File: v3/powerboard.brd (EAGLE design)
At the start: 100 x 80 mm, 17 parts, among them U1 TPS61088VQFN20

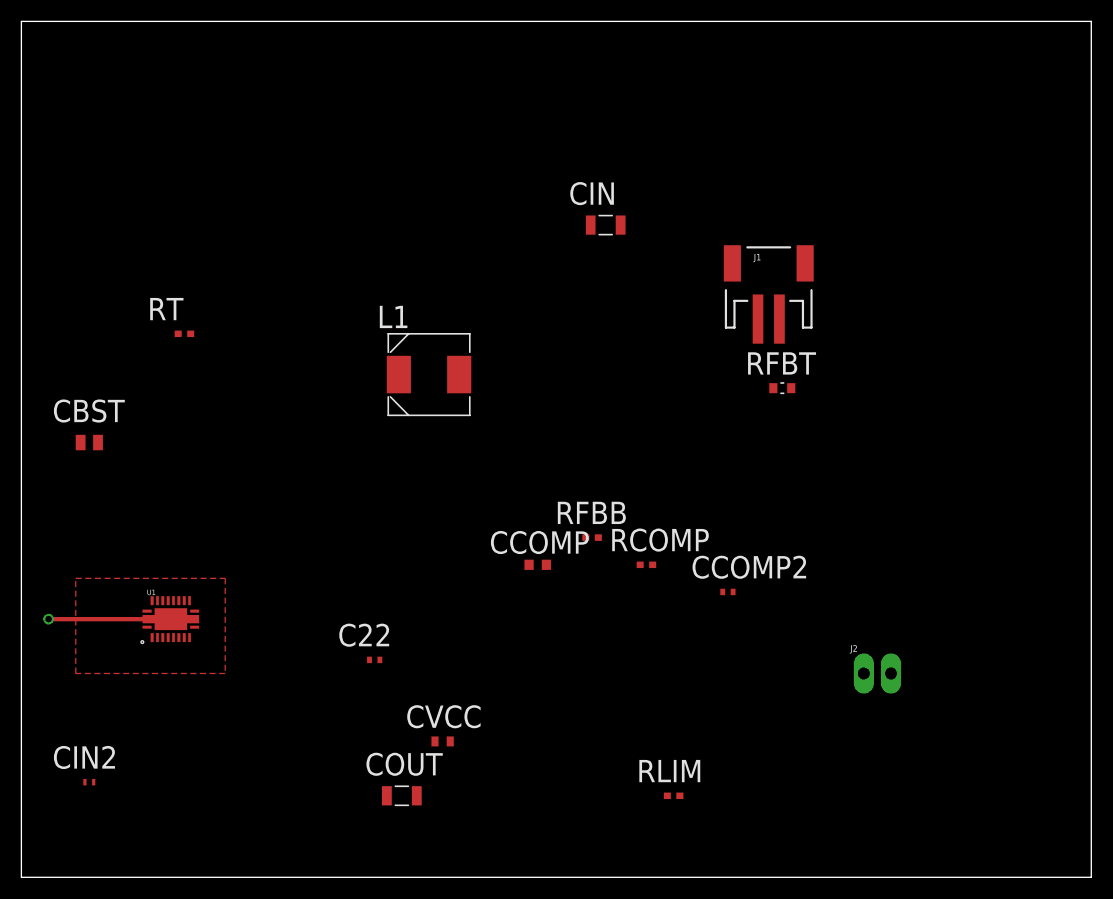
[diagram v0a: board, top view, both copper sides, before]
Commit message: Progress on 6v eval board.
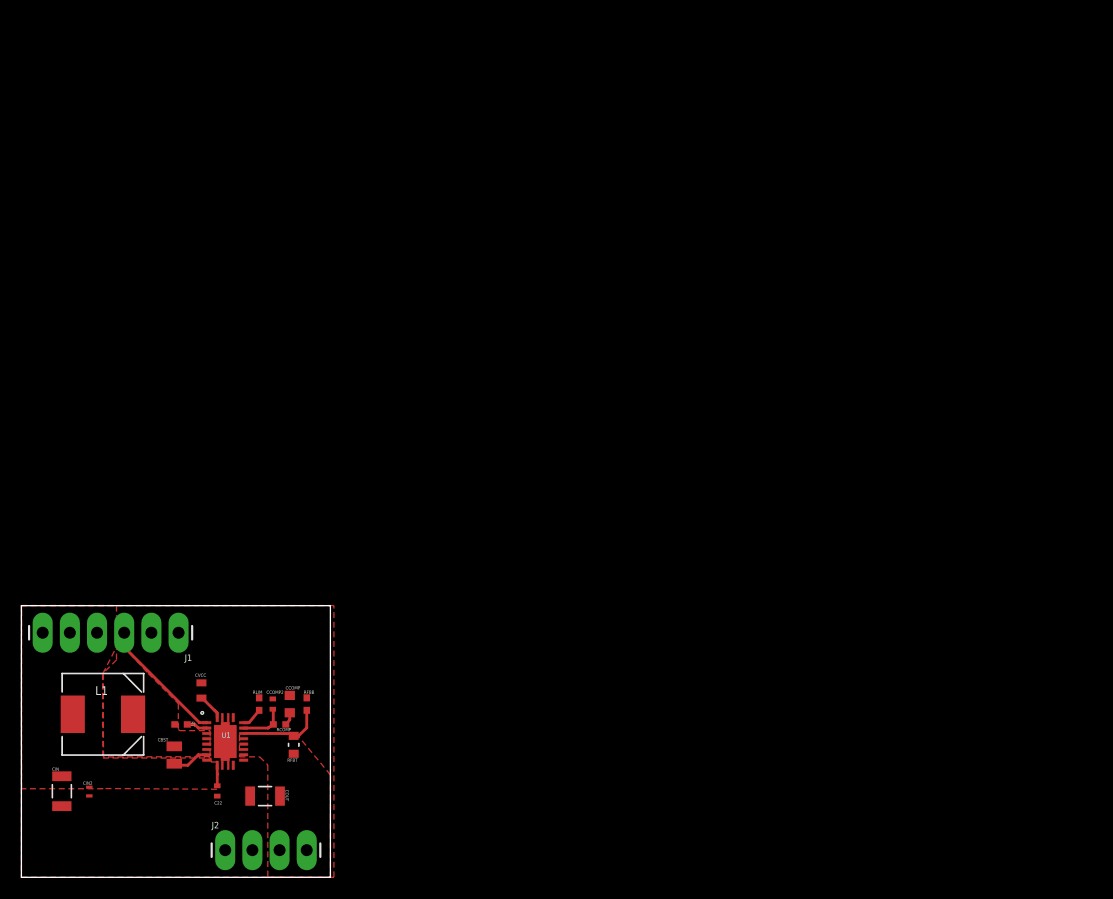
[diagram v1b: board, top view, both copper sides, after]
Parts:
- J1: device SparkFun-Connectors:JST-2-SMD -> SparkFun-Connectors:1X06_LONGPADS
- J2: device SparkFun-Connectors:1X02_LONGPADS -> SparkFun-Connectors:1X04_LONGPADS
- moved CIN 73.4 mm to (3.78, 8.05), turned to 90 degrees
- moved J1 64.3 mm to (14.7, 22.9), turned to 180 degrees
- moved J2 61.9 mm to (19.1, 2.54)
- moved RFBT 56.5 mm to (25.5, 12.4), turned to 90 degrees
- moved L1 44.0 mm to (7.62, 15.2), turned to 180 degrees
- moved CCOMP2 43.8 mm to (23.5, 16.2), turned to 270 degrees
- moved RLIM 39.7 mm to (22.2, 16.2), turned to 90 degrees
- moved RCOMP 37.4 mm to (24.1, 14.3)
- moved RT 36.5 mm to (14.9, 14.3), turned to 180 degrees
- moved RFBB 30.9 mm to (26.7, 16.2), turned to 270 degrees
- moved CBST 30.3 mm to (14.3, 11.4), turned to 90 degrees
- moved CCOMP 26.6 mm to (25.1, 16.2), turned to 270 degrees
- moved CVCC 23.0 mm to (16.8, 17.5), turned to 90 degrees
- moved C22 19.1 mm to (18.3, 8.07), turned to 90 degrees
- moved COUT 12.8 mm to (22.8, 7.59)
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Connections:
- net N$3 renamed FSW
- net N$4 renamed FB
- new net EN: J1.3, U1.P$2
- net GND: now also J1.2, J2.1, U1.P$22, U1.P$23, U1.P$24
- net VCC: no longer U1.P$2
- net VIN: now also J1.4, J1.5, J1.6; no longer J1.2
- net VOUT: now also J2.3, J2.4; no longer J2.1
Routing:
- net EN: track 0.00 -> 12.0 mm
- net GND: track 11.4 -> 0.00 mm, vias 1 -> 0
- net FB: track 0.00 -> 7.92 mm
- net COMP: track 0.00 -> 4.32 mm
- net BOOT: track 0.00 -> 3.50 mm
- net VCC: track 0.00 -> 2.48 mm
- net ILIM: track 0.00 -> 2.00 mm
- net FSW: track 0.00 -> 1.97 mm
- net SS: track 0.00 -> 1.92 mm
- net N$1: track 0.00 -> 1.23 mm
- added copper zone on layer 1, net SW
- added copper zone on layer 1, net VIN
- added copper zone on layer 1, net VOUT
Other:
- board size 100 x 80 mm -> 28.9 x 25.4 mm
